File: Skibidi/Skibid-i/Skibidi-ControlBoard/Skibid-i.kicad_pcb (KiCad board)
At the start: 2 copper layers, 128.7 x 66.8 mm, 60 parts, among them IC1 TEENSY_4.1, J10 Screw_Terminal_01x03, J12 Screw_Terminal_01x03, J13 P78E05-1000, J14 Battery, J15 Conn_01x03_Pin, J16 Conn_01x02_Pin, J17 Conn_01x08_Pin, J18 SparkIN, J19 SparkOUT, J2 Screw_Terminal_01x03, J20 Screw_Terminal_01x03, J21 Motor1, J22 Motor2, J3 Screw_Terminal_01x03, J4 Screw_Terminal_01x03, J5 Screw_Terminal_01x03, J6 Screw_Terminal_01x03, J7 Screw_Terminal_01x03, J8 Screw_Terminal_01x03, J9 Screw_Terminal_01x03, Q1 WL-OCPT_SERIES_357, Q2 WL-OCPT_SERIES_357, Q3 WL-OCPT_SERIES_357, Q4 WL-OCPT_SERIES_357, Q5 WL-OCPT_SERIES_357, Q6 WL-OCPT_SERIES_357, Q7 WL-OCPT_SERIES_357, SW2 210-4MS

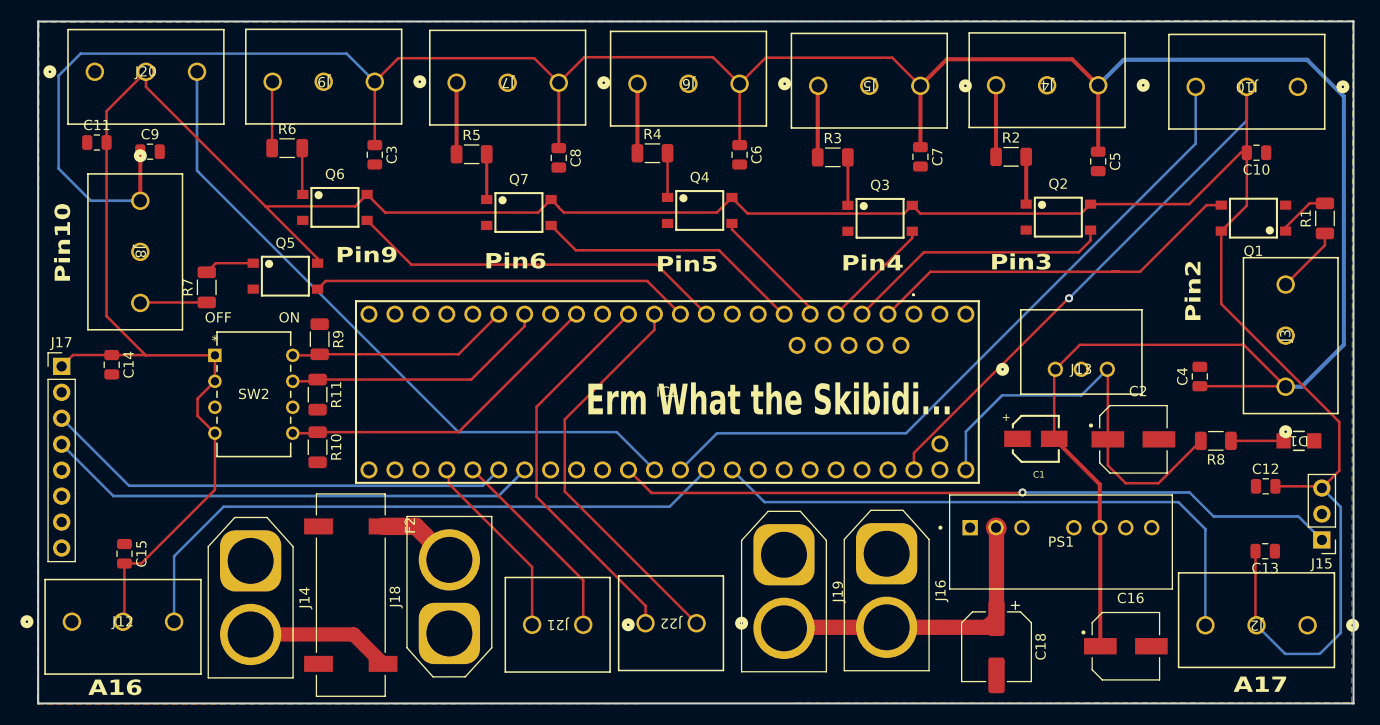
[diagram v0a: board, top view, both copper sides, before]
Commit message: erm
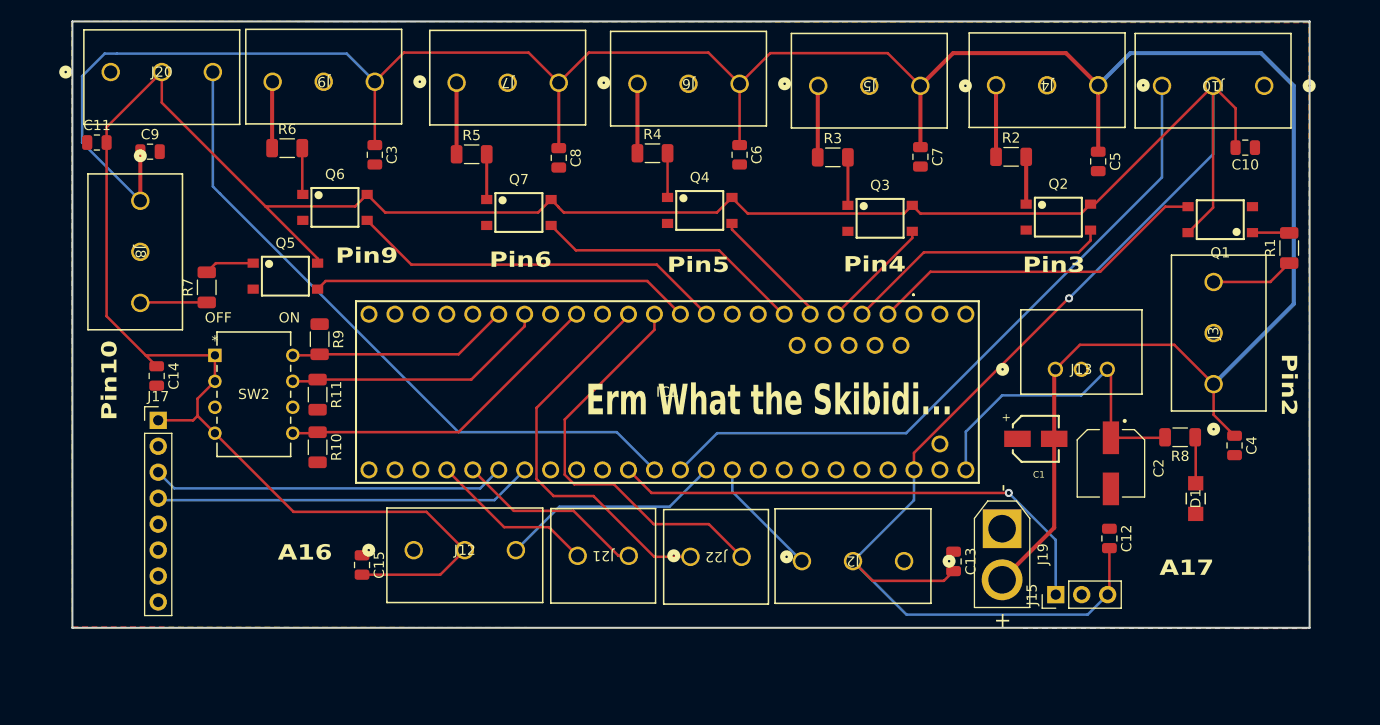
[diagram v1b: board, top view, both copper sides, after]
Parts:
- removed C16: 22uF, askibidi:Ecap
- removed C18: 100uF, Capacitor_SMD:CP_Elec_6.3x5.4
- removed F2: 3587, askibidi:Fusemount
- removed J14: Battery, Connector_AMASS:AMASS_XT60-F_1x02_P7.20mm_Vertical
- removed J16: Conn_01x02_Pin, Connector_AMASS:AMASS_XT60-F_1x02_P7.20mm_Vertical
- removed J18: SparkIN, Connector_AMASS:AMASS_XT60-F_1x02_P7.20mm_Vertical
- removed PS1: RSO-4812S_H2, askibidi:12vConvertor
- J19: value SparkOUT -> 12V; footprint Connector_AMASS:AMASS_XT60-F_1x02_P7.20mm_Vertical -> Connector_AMASS:AMASS_XT30U-F_1x02_P5.0mm_Vertical
- moved J2 40.0 mm to (228.5, 83.6)
- moved J12 34.2 mm to (180.5, 82.6)
- moved C13 30.5 mm to (233.3, 83.7), turned to -90 degrees
- moved J15 26.6 mm to (243.3, 86.9), turned to 90 degrees
- moved C15 23.3 mm to (175.4, 84.0)
- moved J19 21.5 mm to (238.1, 80.5)
- moved C12 16.1 mm to (248.6, 81.4), turned to -90 degrees
- moved D1 11.6 mm to (257.1, 77.5), turned to 90 degrees
- moved J17 10.8 mm to (155.5, 69.8)
- moved J21 8.09 mm to (201.6, 83.1)
- moved J22 7.85 mm to (212.6, 83.2)
- moved C4 7.56 mm to (260.9, 72.3), turned to -90 degrees
- moved J3 7.05 mm to (258.8, 66.3)
- moved R1 4.55 mm to (266.2, 53.0)
- moved C14 4.54 mm to (155.3, 65.5)
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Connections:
- J19 pad 2: +48V -> +12V
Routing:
- net LN4: track 58.1 -> 11.8 mm
- net LN3: track 62.0 -> 21.9 mm
- net +48V: track 30.1 -> 0.00 mm
- net +12V: track 287.4 -> 263.0 mm
- net Start: track 70.8 -> 50.1 mm
- net Net-(J14-Pin_2): track 14.2 -> 0.00 mm
- net SCL: track 46.2 -> 34.7 mm
- net SDA: track 48.5 -> 37.2 mm
- net +5V: track 41.1 -> 32.3 mm
- net Net-(J18-Pin_2): track 7.85 -> 0.00 mm
- net +3.3V: track 340.9 -> 347.7 mm
- net Dis1: track 37.8 -> 33.7 mm
- net BDC22: track 18.6 -> 16.3 mm
- net Net-(Q1-Pad1): track 5.19 -> 3.61 mm
- net OM1: track 6.88 -> 8.17 mm
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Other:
- board size 128.7 x 66.8 mm -> 121.1 x 59.4 mm
